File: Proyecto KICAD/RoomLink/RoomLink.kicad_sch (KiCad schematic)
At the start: 6 parts, among them J1 TBP04R12-500-02BE, J2 TBP04R12-500-02BE, J3 TBP04R12-500-02BE, J4 TBP04R12-500-03GR, J5 TBP04R12-500-08GR, J6 TBP04R12-500-08GR

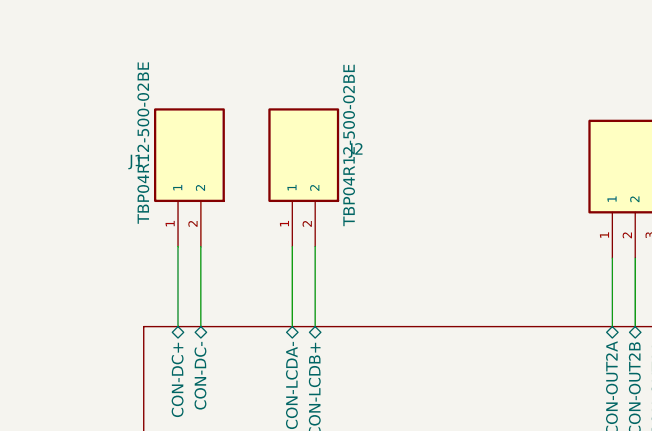
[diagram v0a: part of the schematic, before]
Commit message: Raymundo
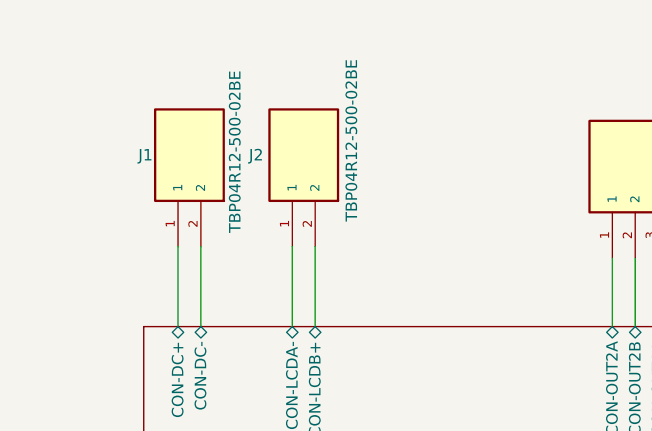
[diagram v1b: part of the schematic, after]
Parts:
- J4: footprint CUI_TBP04R12-500-03GR -> TBP04R12-500-03GR:CUI_TBP04R12-500-03GR
- J5, J6: footprint CUI_TBP04R12-500-08GR -> TBP04R12-500-08GR:CUI_TBP04R12-500-08GR
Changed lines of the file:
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@@
       (effects (font (size 1.27 1.27)) (justify right))
     )
-    (property "Footprint" "CUI_TBP04R12-500-08GR" (at 167.64 58.42 0)
+    (property "Footprint" "TBP04R12-500-08GR:CUI_TBP04R12-500-08GR" (at 167.64 58.42 0)
       (effects (font (size 1.27 1.27)) (justify left bottom) hide)
     )
@@
       (effects (font (size 1.27 1.27)) (justify left))
     )
-    (property "Footprint" "CUI_TBP04R12-500-03GR" (at 129.54 121.92 0)
+    (property "Footprint" "TBP04R12-500-03GR:CUI_TBP04R12-500-03GR" (at 129.54 121.92 0)
       (effects (font (size 1.27 1.27)) (justify left bottom) hide)
     )
@@
       (effects (font (size 1.27 1.27)) (justify left))
     )
-    (property "Footprint" "CUI_TBP04R12-500-08GR" (at 170.18 121.92 0)
+    (property "Footprint" "TBP04R12-500-08GR:CUI_TBP04R12-500-08GR" (at 170.18 121.92 0)
       (effects (font (size 1.27 1.27)) (justify left bottom) hide)
     )
@@
   (symbol (lib_id "TBP04R12-500-02BE:TBP04R12-500-02BE") (at 124.46 57.15 90) (unit 1)
     (in_bom yes) (on_board yes) (dnp no)
-    (property "Reference" "J2" (at 130.81 56.515 90)
+    (property "Reference" "J2" (at 119.634 57.15 90)
       (effects (font (size 1.27 1.27)) (justify right))
     )
-    (property "Value" "TBP04R12-500-02BE" (at 130.81 46.99 0)
+    (property "Value" "TBP04R12-500-02BE" (at 131.064 46.482 0)
       (effects (font (size 1.27 1.27)) (justify right))
     )
@@
   (symbol (lib_id "TBP04R12-500-02BE:TBP04R12-500-02BE") (at 111.76 57.15 90) (unit 1)
     (in_bom yes) (on_board yes) (dnp no)
-    (property "Reference" "J1" (at 107.95 57.785 90)
+    (property "Reference" "J1" (at 108.966 57.15 90)
       (effects (font (size 1.27 1.27)) (justify left))
     )
-    (property "Value" "TBP04R12-500-02BE" (at 107.95 64.77 0)
+    (property "Value" "TBP04R12-500-02BE" (at 118.11 65.786 0)
       (effects (font (size 1.27 1.27)) (justify left))
     )
